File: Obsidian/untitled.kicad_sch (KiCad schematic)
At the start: 72 parts, among them U12 LP5951MF-3.0/NOPB, U13 LM336M-2.5, U14 DAC8550IDGK, U15 DAC8550IDGK, U16 CDCM61004RHB, U3 Si5351A-B-GT, Y1 OSC_25MHZ_RAKON_IVT3205CR, Y2 VM53S3-25.000-2.5/-30+75, Y3 OSC_20MHZ_IQD_LFVCXO026156, Y6 XTAL_25MHZ_TXC_8Y-25.000MAAJ-T

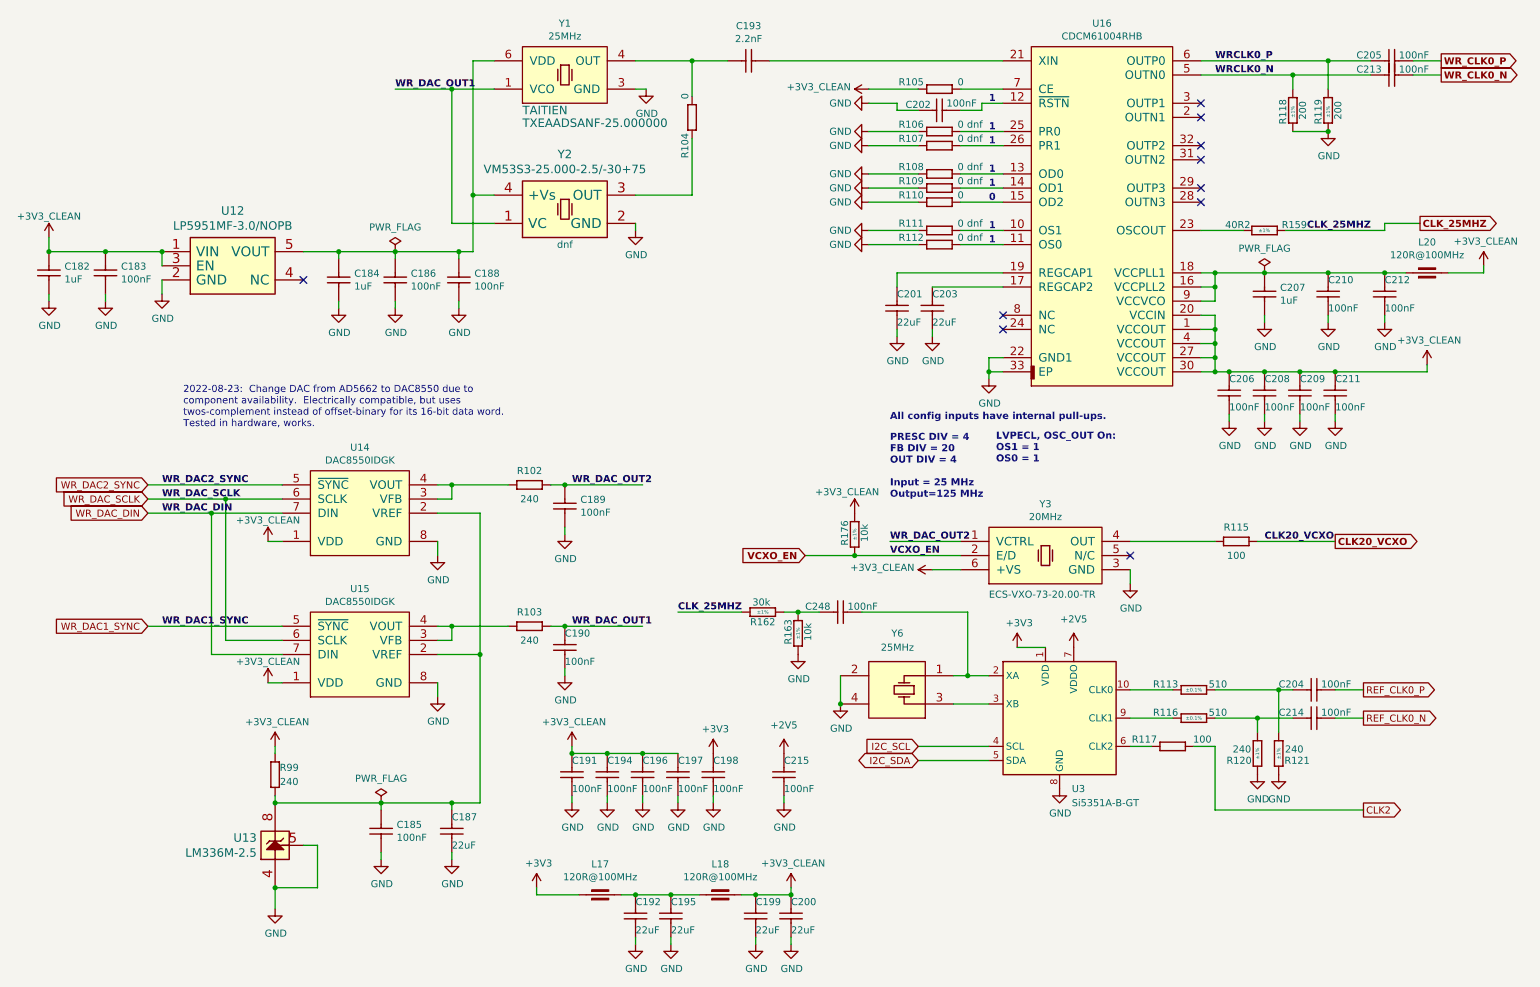
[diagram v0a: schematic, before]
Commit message: revison v1.1.0 ready to review
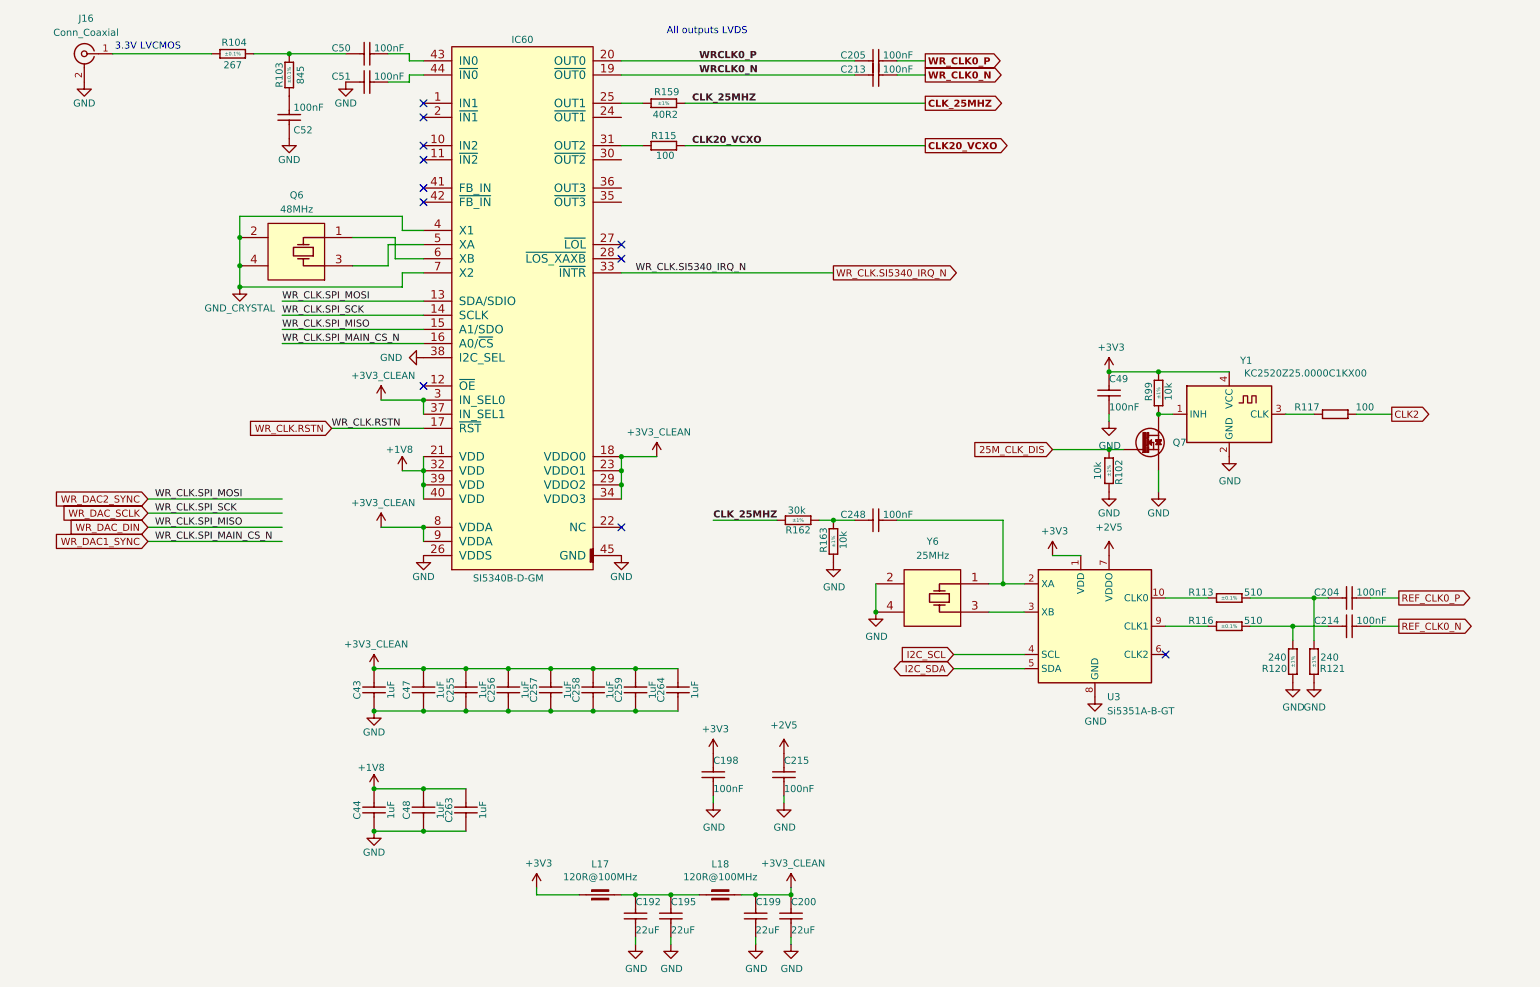
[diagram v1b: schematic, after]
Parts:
- removed C182, C184, C207: CC0402_1UF_16V_10%_X5R, Capacitors SMD:CAPC1005X55N, symbol Capacitors_SMD:CC0402_1UF_16V_10%_X5R
- removed C183, C185, C186, C188, C189, C190, C191, C194, C196, C197, C206, C208, C209, C210, C211, C212: CC0201_100NF_6.3V_10%_X5R, Capacitors SMD:CAPC0603X33N, symbol Capacitors_SMD:CC0201_100NF_6.3V_10%_X5R
- removed C187, C201, C203: CC0603_22UF_6.3V_20%_X5R, CAPC1709X100N, symbol Capacitors_SMD:CC0603_22UF_6.3V_20%_X5R
- removed C193: CC0402_2.2NF_50V_10%_X7R, Capacitors SMD:CAPC1005X55N, symbol Capacitors_SMD:CC0402_2.2NF_50V_10%_X7R
- removed C202: CC0402_100NF_50V_10%_X7R, Capacitors SMD:CAPC1005X55N, symbol Capacitors SMD:CC0402_100NF_50V_10%_X7R
- removed L20: IND0603_MURATA_BLM18SG121TN1D, INDC1608X65N, symbol Inductors_SMD:IND0603_MURATA_BLM18SG121TN1D
- removed R102, R103, R99: R0402_240R_1%_0.0625W_100PPM, Resistors SMD:RESC1005X40N, symbol Resistors_SMD:R0402_240R_1%_0.0625W_100PPM
- removed R104, R105, R106, R107, R108, R109, R110, R111, R112: R0402_0R_JUMPER, RESC1005X40N, symbol Resistors_SMD:R0402_0R_JUMPER
- removed R118, R119: R0402_200R_1%_0.0625W_100PPM, Resistors SMD:RESC1005X40N, symbol Resistors SMD:R0402_200R_1%_0.0625W_100PPM
- removed R176: R0402_10K_1%_0.0625W_100PPM, Resistors SMD:RESC1005X40N, symbol Resistors SMD:R0402_10K_1%_0.0625W_100PPM
- removed U12: LP5951MF-3.0/NOPB, ICs And Semiconductors SMD:SOT95P284X122-5N, symbol marble_misc:LP5951-clocks-SchDoc-cache
- removed U13: LM336M-2.5, ICs And Semiconductors SMD:SOIC127P600X175-8N, symbol marble_misc:LM336M-2.5-clocks-SchDoc-cache
- removed U14, U15: DAC8550IDGK, ICs And Semiconductors SMD:SOP65P490X110-8N, symbol Analog_&_Interface:DAC8550IDGK
- removed U16: CDCM61004RHB, ICs And Semiconductors SMD:QFN50P500X500X100-33N-S355, symbol Logic:CDCM61004RHB
- removed Y1: OSC_25MHZ_RAKON_IVT3205CR, ICs And Semiconductors SMD:OSC_ABRACON_ASEMPC, symbol Crystals_&_Oscillators:OSC_25MHZ_RAKON_IVT3205CR
- removed Y2: VM53S3-25.000-2.5/-30+75, ICs And Semiconductors SMD:OSCCC320X500X160-4N, symbol marble_misc:Oscillator_1VC_2GND_3OUT_4+Vs-clocks-SchDoc-cache
- removed Y3: OSC_20MHZ_IQD_LFVCXO026156, ICs And Semiconductors SMD:OSC_IQD_CFPV-45, symbol Crystals_&_Oscillators:OSC_20MHZ_IQD_LFVCXO026156
- added C255, C256, C257, C258, C259, C263, C264, C43, C44, C47, C48: CC0402_1UF_25V_10%_X5R, Capacitors SMD:CAPC1005X55N, symbol Capacitors SMD:CC0402_1UF_25V_10%_X5R
- added C49: CC0201_100NF_6.3V_10%_X5R, Capacitors SMD:CAPC0603X33N, symbol Capacitors_SMD:CC0201_100NF_6.3V_10%_X5R
- added C50, C51, C52: CC0402_100NF_50V_10%_X7R, Capacitors SMD:CAPC1005X55N, symbol Capacitors SMD:CC0402_100NF_50V_10%_X7R
- added IC60: SI5340B-D-GM, ICs And Semiconductors SMD:QFN50P700X700X90-45N-S530, symbol Analog & Interface:SI5340B-D-GM
- added J16: Conn_Coaxial, Connector_Coaxial:SMA_Amphenol_901-144_Vertical, symbol Connector:Conn_Coaxial
- added Q6: XTAL_48MHZ_KYOCERA_CX3225SB48000D0FPJC1, ICs And Semiconductors SMD:XTAL_KYOCERA_CX3225SB, symbol Crystals & Oscillators:XTAL_48MHZ_KYOCERA_CX3225SB48000D0FPJC1
- added Q7: BSS138LT1G, ICs And Semiconductors SMD:SOT95P240X110-3N, symbol Transistors:BSS138LT1G
- added R102, R99: R0402_10K_1%_0.0625W_100PPM, Resistors SMD:RESC1005X40N, symbol Resistors SMD:R0402_10K_1%_0.0625W_100PPM
- added R103: R0603_845R_0.1%_0.063W_10PPM, Resistors SMD:RESC1608X55N, symbol Resistors SMD old:R0603_845R_0.1%_0.063W_10PPM
- added R104: R0603_267R_0.1%_0.063W_10PPM, Resistors SMD:RESC1608X55N, symbol Resistors SMD old:R0603_267R_0.1%_0.063W_10PPM
- added Y1: KC2520Z25.0000C1KX00, Oscillator:Oscillator_SMD_Kyocera_KC2520Z-4Pin_2.5x2.0mm, symbol Oscillator:KC2520Z
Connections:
- net +3V3: now also C49.1, R99.2, Y1.4 (VCC)
- net +3V3_CLEAN: now also C255.2, C256.2, C257.2, C258.2, C259.2, C264.2, C43.2, C47.2, IC60.18 (VDDO0), IC60.23 (VDDO1), IC60.29 (VDDO2), IC60.3 (IN_SEL0), IC60.34 (VDDO3), IC60.37 (IN_SEL1), IC60.8 (VDDA), IC60.9 (VDDA)
- net GND: now also C255.1, C256.1, C257.1, C258.1, C259.1, C263.1, C264.1, C43.1, C44.1, C47.1, C48.1, C49.2, C51.2, C52.2, IC60.26 (VDDS), IC60.38 (I2C_SEL), IC60.45 (GND), J16.2 (Ext), Q7.2 (S), R102.1, Y1.2 (GND)
- net WRCLK0_N: now also IC60.19 (~{OUT0})
- net WRCLK0_P: now also IC60.20 (OUT0)
- net WR_DAC1_SYNC: now also IC60.16 (A0/~{CS})
- net WR_DAC2_SYNC: now also IC60.13 (SDA/SDIO)
- net WR_DAC_DIN: now also IC60.15 (A1/SDO)
- net WR_DAC_SCLK: now also IC60.14 (SCLK)
- net at R159.1: now also IC60.25 (OUT1)
- net at U3.6 (CLK2): no longer R117.1
- net at R115.1: now also IC60.31 (OUT2)
- new net: C50.1, IC60.43 (IN0)
- new net: C50.2, R103.2, R104.2
- new net: Q7.3 (D), R99.1, Y1.1 (INH)
- new net: IC60.6 (XB), Q6.1 (X)
- new net: IC60.5 (XA), Q6.3 (X)
- new net: C51.1, IC60.44 (~{IN0})
- new net: C52.1, R103.1
- new net: J16.1 (In), R104.1
- new net: R117.1, Y1.3 (CLK)
- new net +1V8: C263.2, C44.2, C48.2, IC60.21 (VDD), IC60.32 (VDD), IC60.39 (VDD), IC60.40 (VDD)
- new net 25M_CLK_DIS: Q7.1 (G), R102.2
- new net GND_CRYSTAL: IC60.4 (X1), IC60.7 (X2), Q6.2 (GND), Q6.4 (GND)
- new net WR_CLK.RSTN: IC60.17 (~{RST})
- new net WR_CLK.SI5340_IRQ_N: IC60.33 (~{INTR})
- no-connect marks 10 -> 11
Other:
- note added: "3.3V LVCMOS"
- note added: "All outputs LVDS"
- note removed: "0"
- note removed: "1"
- note removed: "2022-08-23: Change DAC from AD5662 to DAC8550 due to component availability. Electrically compatible, but uses twos-complement instead of offset-binary for its 16-bit data word. Tested in hardware, works."
- note removed: "All config inputs have internal pull-ups."
- note removed: "LVPECL, OSC_OUT On: OS1 = 1 OS0 = 1"
- note removed: "PRESC DIV = 4 FB DIV = 20 OUT DIV = 4 Input = 25 MHz Output=125 MHz"
- moved on the sheet: C204, C205, C213, C214, C248, R113, R115, R116, R117, R120, R121, R159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
